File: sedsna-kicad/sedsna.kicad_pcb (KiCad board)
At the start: 4 copper layers, 42 x 99 mm, 50 parts, among them J1 Conn_01x03, J10 Conn_01x03, J11 BAT1, J2 Conn_01x03, J3 Servos_Rudder/Elevator, J4 L_Aileron, J5 USB4105-GF-A, J6 R_Aileron, J7 Prop, J9 Conn_01x03, U2 ESP32-C3, U4 Magnetometer, U5 IMU, U6 LDL1117S33R

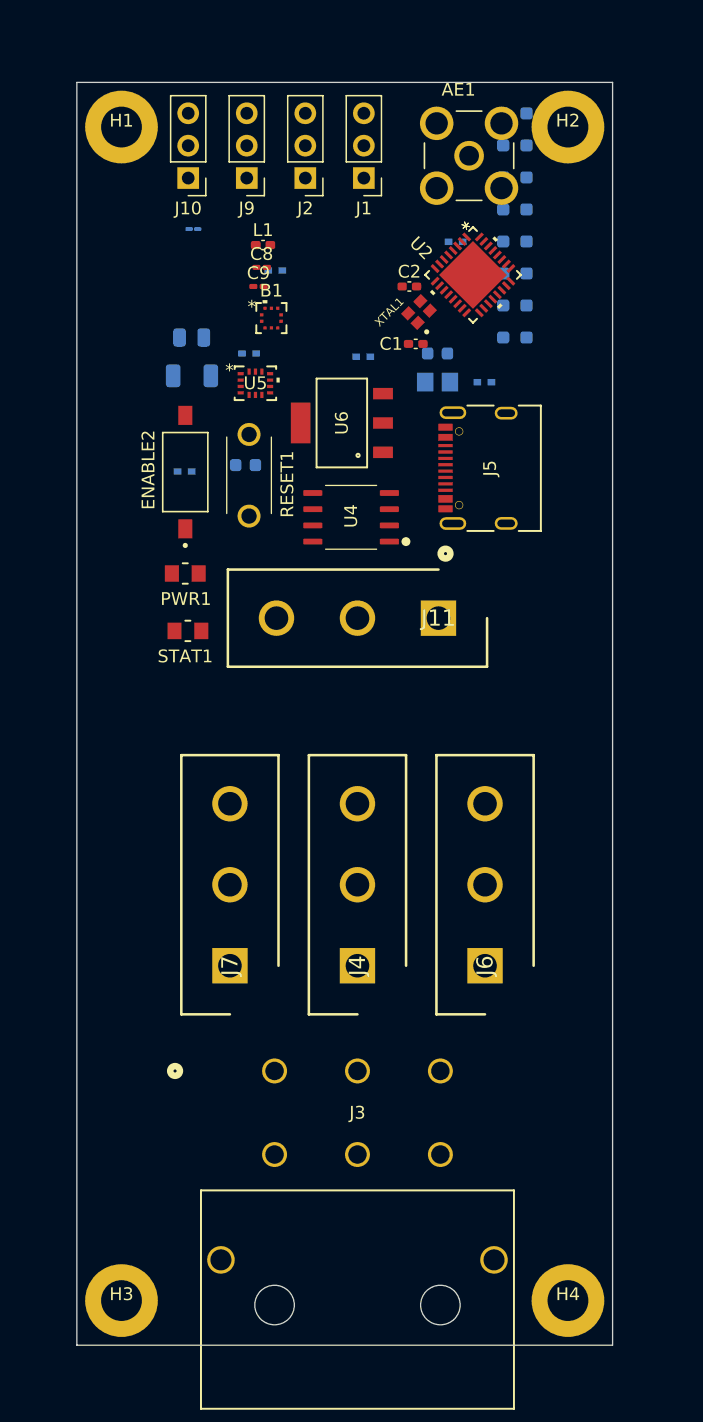
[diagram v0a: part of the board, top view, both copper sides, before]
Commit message: Finished layout
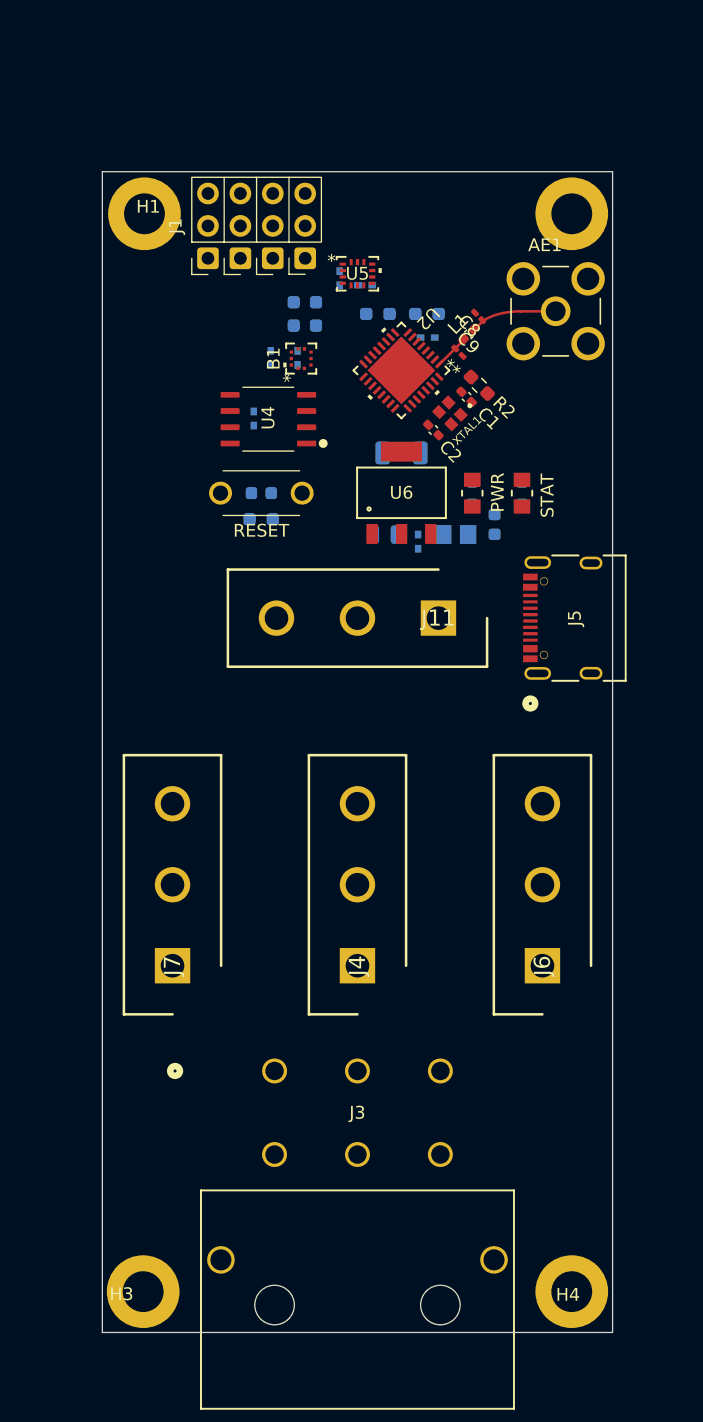
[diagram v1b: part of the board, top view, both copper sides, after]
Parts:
- removed ENABLE2: Enable Switch, TR3_V1:SW_DS04-254-2-01BK-SMT
- removed J10, J2, J9: Conn_01x03, Connector_PinHeader_2.54mm:PinHeader_1x03_P2.54mm_Vertical
- C7: footprint Capacitor_SMD:C_01005_0402Metric_Pad0.57x0.30mm_HandSolder -> TR3_V1:CAP_CL05_SAM
- J1: value Conn_01x03 -> ~; footprint Connector_PinHeader_2.54mm:PinHeader_1x03_P2.54mm_Vertical -> sedsna:Conn_04x03
- R2: moved to F.Cu
- moved R7 35.4 mm to (109.0, 76.8), turned to 0 degrees
- moved STAT 28.3 mm to (129.4, 74.7), turned to 90 degrees
- moved PWR 23.4 mm to (125.5, 74.7), turned to 90 degrees
- moved C19 21.8 mm to (122.0, 62.5)
- moved C5 21.6 mm to (118.7, 78.0), turned to 0 degrees
- moved R2 21.5 mm to (126.0, 66.2), turned to -45 degrees
- moved R8 20.4 mm to (111.5, 60.6), turned to 90 degrees
- moved R16 20.0 mm to (125.5, 74.7), turned to 90 degrees
- moved R12 17.6 mm to (113.2, 60.6), turned to 90 degrees
- moved L1 17.6 mm to (125.2, 62.2), turned to 45 degrees
- moved C6 17.5 mm to (120.0, 71.5)
- moved C8 17.4 mm to (126.0, 60.9), turned to 135 degrees
- moved R17 17.2 mm to (129.4, 74.7), turned to 90 degrees
- moved C9 16.5 mm to (124.5, 63.6), turned to -45 degrees
- moved C7 15.6 mm to (108.4, 68.8), turned to -90 degrees
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- renumbered PWR1 to PWR, RESET1 to RESET, STAT1 to STAT
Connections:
- C4 pad 1: +7.4V -> +6.6V
- C5 pad 2: +7.4V -> +6.6V
- FB1 pad 2: +7.4V -> +6.6V
- J11 pad 1: +7.4V -> +6.6V
- J11 pad 3: +7.4V -> unconnected-(J11-Pin_3-Pad3)
- J3 pad 2: +7.4V -> +6.6V
- J3 pad 5: +7.4V -> +6.6V
- J4 pad 2: +7.4V -> +6.6V
- J5 pad A6: /USB_D+ -> Earth
- J5 pad B6: /USB_D+ -> Earth
- J6 pad 2: +7.4V -> +6.6V
- R7 pad 1: Net-(ENABLE2-Pad1) -> +3.3V
- U2 pad 26: /USB_D+ -> Earth
- U2 pad 27: unconnected-(U2-U0RXD-Pad27) -> Earth
- U6 pad 3: +7.4V -> +6.6V
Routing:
- net Net-(AE1-Pad1): track 0.00 -> 3.77 mm
- net /ANT: track 0.00 -> 2.73 mm
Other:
- board size 42 x 99 mm -> 40 x 91 mm
